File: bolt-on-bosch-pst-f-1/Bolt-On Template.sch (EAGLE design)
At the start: 10 parts

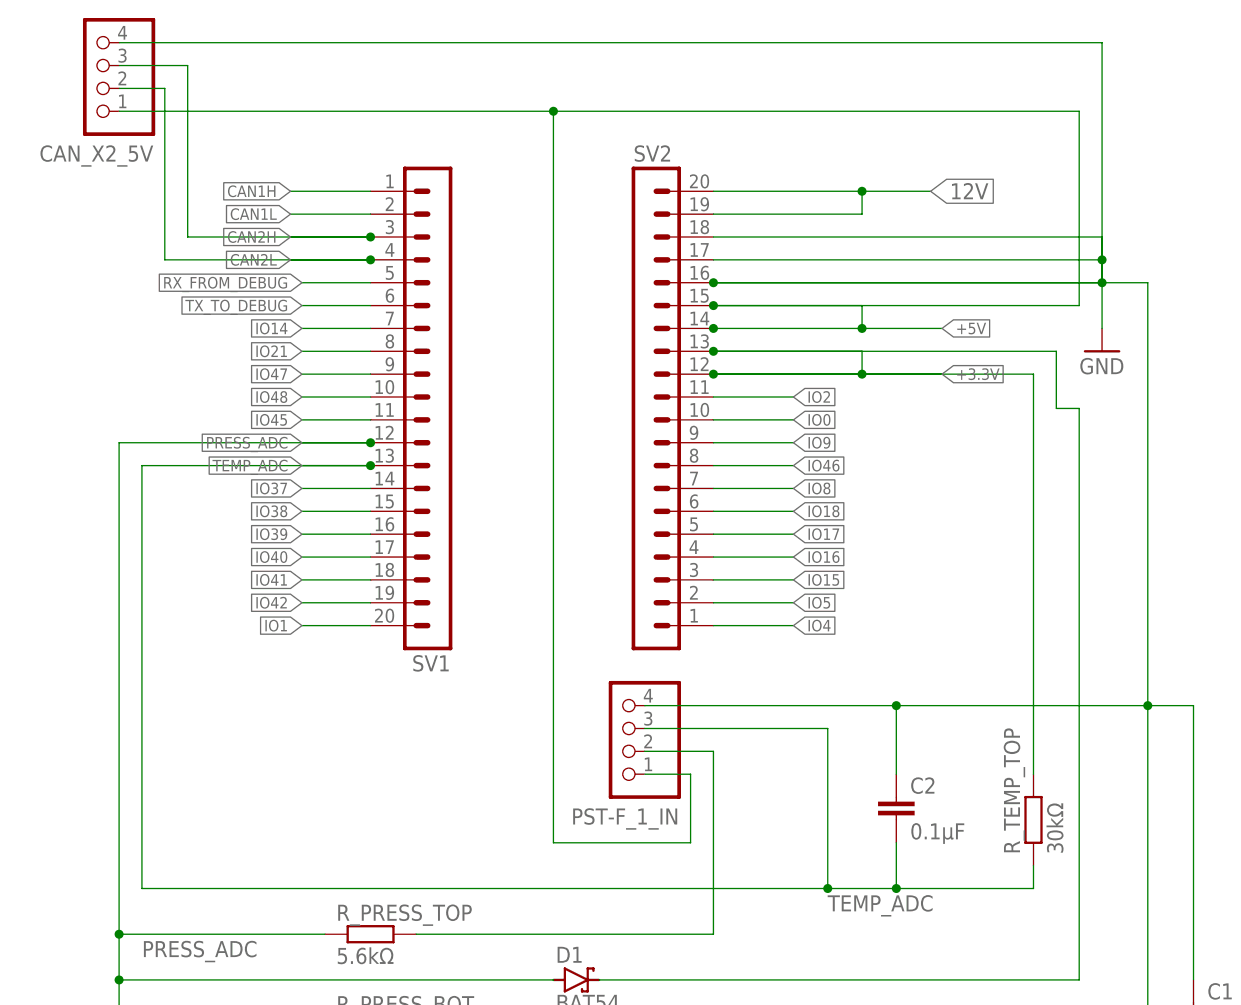
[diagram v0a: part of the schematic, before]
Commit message: cleanup board design
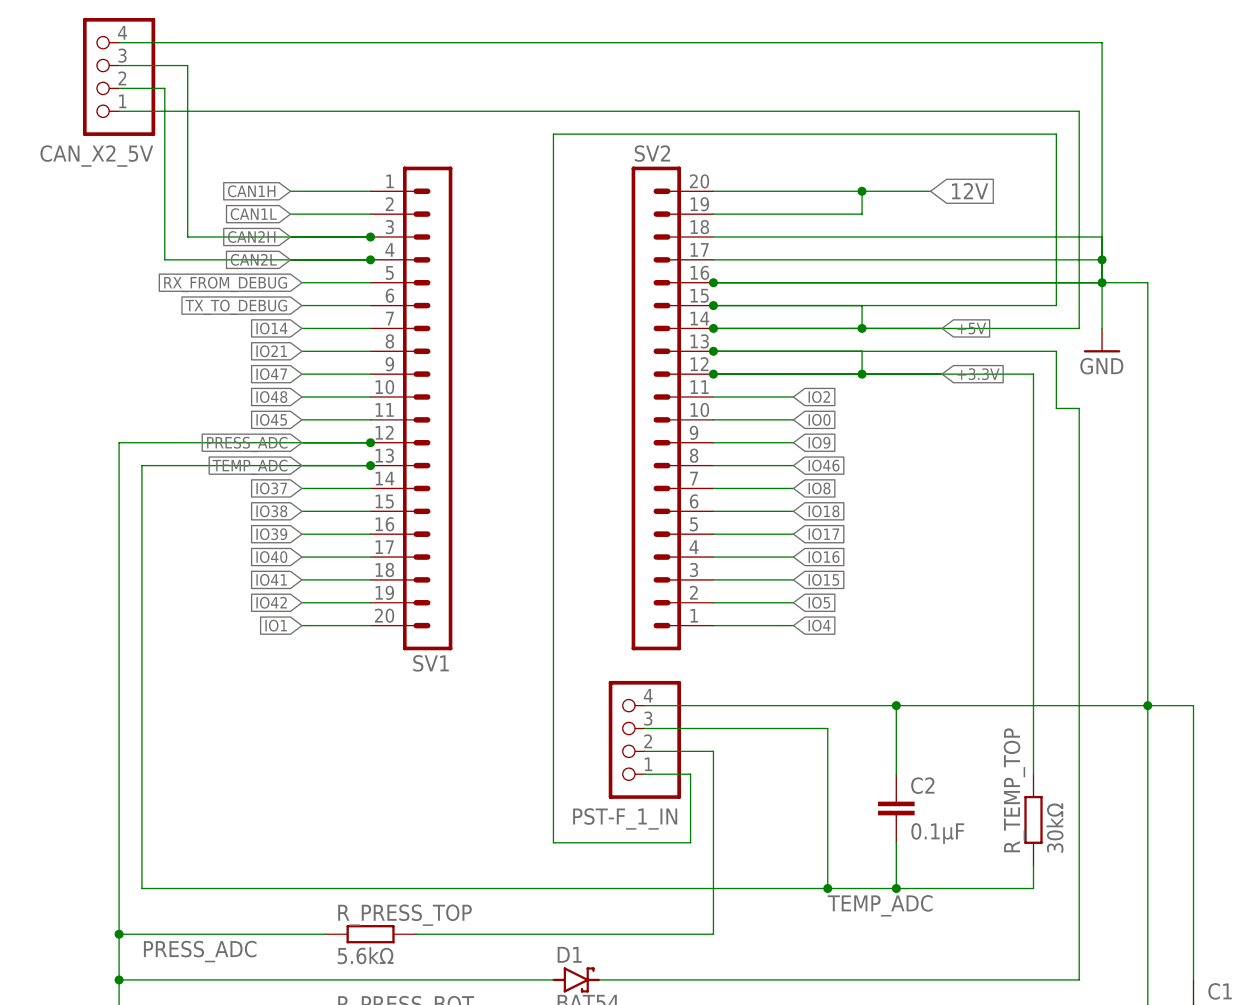
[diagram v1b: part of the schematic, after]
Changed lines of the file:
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@@
 <wire x1="210.82" y1="88.9" x2="210.82" y2="81.28" width="0.1524" layer="91"/>
 <wire x1="210.82" y1="81.28" x2="195.58" y2="81.28" width="0.1524" layer="91"/>
-<wire x1="195.58" y1="81.28" x2="195.58" y2="162.56" width="0.1524" layer="91"/>
+<wire x1="195.58" y1="81.28" x2="195.58" y2="160.02" width="0.1524" layer="91"/>
 <wire x1="229.87" y1="138.43" x2="238.76" y2="138.43" width="0.1524" layer="91"/>
 <pinref part="SV2" gate="1" pin="15"/>
@@
 <wire x1="213.36" y1="138.43" x2="229.87" y2="138.43" width="0.1524" layer="91"/>
 <label x="238.76" y="138.43" size="1.27" layer="95" xref="yes"/>
-<wire x1="254" y1="162.56" x2="254" y2="140.97" width="0.1524" layer="91"/>
-<wire x1="254" y1="140.97" x2="213.36" y2="140.97" width="0.1524" layer="91"/>
 <junction x="213.36" y="138.43"/>
+<pinref part="CAN_X2_5V" gate="G$1" pin="1"/>
+<wire x1="254" y1="162.56" x2="147.32" y2="162.56" width="0.1524" layer="91"/>
+<pinref part="PST-F_1_IN" gate="G$1" pin="1"/>
+<wire x1="210.82" y1="88.9" x2="205.74" y2="88.9" width="0.1524" layer="91"/>
+<wire x1="254" y1="162.56" x2="254" y2="138.43" width="0.1524" layer="91"/>
+<wire x1="254" y1="138.43" x2="213.36" y2="138.43" width="0.1524" layer="91"/>
+<wire x1="195.58" y1="160.02" x2="251.46" y2="160.02" width="0.1524" layer="91"/>
+<wire x1="251.46" y1="160.02" x2="251.46" y2="140.97" width="0.1524" layer="91"/>
+<wire x1="251.46" y1="140.97" x2="213.36" y2="140.97" width="0.1524" layer="91"/>
 <junction x="213.36" y="140.97"/>
-<pinref part="CAN_X2_5V" gate="G$1" pin="1"/>
-<wire x1="254" y1="162.56" x2="195.58" y2="162.56" width="0.1524" layer="91"/>
-<pinref part="PST-F_1_IN" gate="G$1" pin="1"/>
-<wire x1="195.58" y1="162.56" x2="147.32" y2="162.56" width="0.1524" layer="91"/>
-<wire x1="210.82" y1="88.9" x2="205.74" y2="88.9" width="0.1524" layer="91"/>
-<junction x="195.58" y="162.56"/>
 </segment>
 </net>
